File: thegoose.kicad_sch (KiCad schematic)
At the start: 31 parts, among them U1 DRV8848, U2 DRV8848, U3 DRV8848, U4 AP64500SP-13

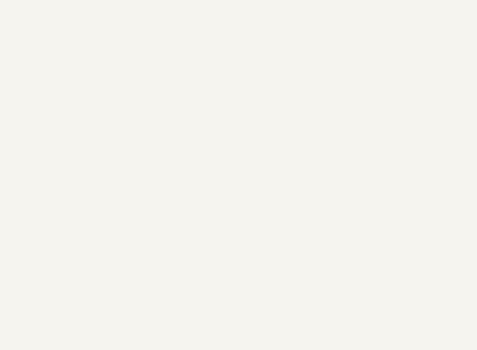
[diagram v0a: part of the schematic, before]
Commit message: Add LCSC part numbers
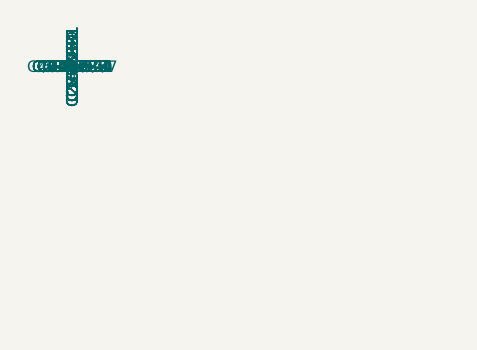
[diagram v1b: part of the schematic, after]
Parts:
- BT1: LCSC Part # (none) -> C98732
- C1: LCSC Part # (none) -> C106837
- C10, C15, C3, C6: LCSC Part # (none) -> C272880
- C11, C14, C4, C7: LCSC Part # (none) -> C344180
- C13, C2, C9: LCSC Part # (none) -> C76638
- C16: LCSC Part # (none) -> C1847101
- ESP32: LCSC Part # (none) -> C82899
- GPIO1: LCSC Part # (none) -> C42431837
- L1: LCSC Part # (none) -> C167779
- M1, M2, M3, M4, M5, M6: LCSC Part # (none) -> C157931
- R25: LCSC Part # (none) -> C844827
- R26: LCSC Part # (none) -> C5200544
- R27: LCSC Part # (none) -> C856785
- R28: LCSC Part # (none) -> C170028
- U1, U2, U3: LCSC Part # (none) -> C2863921
- U4: LCSC Part # (none) -> C2070920
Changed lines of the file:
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@@
 		(on_board yes)
 		(dnp no)
+		(property "LCSC Part #" "C344180")
 		(property "Reference" "C7"
 			(at 145.796 43.942 0)
@@
 		(dnp no)
 		(fields_autoplaced yes)
+		(property "LCSC Part #" "C272880")
 		(property "Reference" "C15"
 			(at 44.45 171.4499 0)
@@
 		(on_board yes)
 		(dnp no)
+		(property "LCSC Part #" "C157931")
 		(property "Reference" "M3"
 			(at 162.56 16.51 90)
@@
 		(on_board yes)
 		(dnp no)
+		(property "LCSC Part #" "C42431837")
 		(property "Reference" "GPIO1"
 			(at 102.362 95.758 0)
@@
 		(dnp no)
 		(fields_autoplaced yes)
+		(property "LCSC Part #" "C167779")
 		(property "Reference" "L1"
 			(at 82.55 158.75 90)
@@
 		(on_board yes)
 		(dnp no)
+		(property "LCSC Part #" "C82899")
 		(property "Reference" "ESP32"
 			(at 47.498 103.632 0)
@@
 		(on_board yes)
 		(dnp no)
+		(property "LCSC Part #" "C344180")
 		(property "Reference" "C11"
 			(at 74.676 43.942 0)
@@
 		(on_board yes)
 		(dnp no)
+		(property "LCSC Part #" "C844827")
 		(property "Reference" "R25"
 			(at 55.88 177.8 90)
@@
 		(on_board yes)
 		(dnp no)
+		(property "LCSC Part #" "C76638")
 		(property "Reference" "C2"
 			(at 225.552 21.844 0)
@@
 		(on_board yes)
 		(dnp no)
+		(property "LCSC Part #" "C2070920")
 		(property "Reference" "U4"
 			(at 64.77 164.592 0)
@@
 		(on_board yes)
 		(dnp no)
+		(property "LCSC Part #" "C5200544")
 		(property "Reference" "R26"
 			(at 101.6 167.64 90)
@@
 		(dnp no)
 		(fields_autoplaced yes)
+		(property "LCSC Part #" "C2863921")
 		(property "Reference" "U3"
 			(at 114.3 46.6246 90)
@@
 		(on_board yes)
 		(dnp no)
+		(property "LCSC Part #" "C98732")
 		(property "Reference" "BT1"
 			(at 39.37 158.75 0)
@@
 		(on_board yes)
 		(dnp no)
+		(property "LCSC Part #" "C157931")
 		(property "Reference" "M2"
 			(at 245.11 16.51 90)
@@
 		(on_board yes)
 		(dnp no)
+		(property "LCSC Part #" "C272880")
 		(property "Reference" "C6"
 			(at 129.794 34.798 0)
@@
 		(on_board yes)
 		(dnp no)
+		(property "LCSC Part #" "C106837")
 		(property "Reference" "C1"
 			(at 16.764 98.806 0)
@@
 		(on_board yes)
 		(dnp no)
+		(property "LCSC Part #" "C272880")
 		(property "Reference" "C10"
 			(at 58.674 34.798 0)
@@
 		(on_board yes)
 		(dnp no)
+		(property "LCSC Part #" "C344180")
 		(property "Reference" "C4"
 			(at 218.186 43.942 0)
@@
 		(on_board yes)
 		(dnp no)
+		(property "LCSC Part #" "C157931")
 		(property "Reference" "M4"
 			(at 172.72 16.51 90)
@@
 		(on_board yes)
 		(dnp no)
+		(property "LCSC Part #" "C157931")
 		(property "Reference" "M5"
 			(at 91.44 16.51 90)
@@
 		(on_board yes)
 		(dnp no)
+		(property "LCSC Part #" "C157931")
 		(property "Reference" "M1"
 			(at 234.95 16.51 90)
@@
 		(on_board yes)
 		(dnp no)
+		(property "LCSC Part #" "C157931")
 		(property "Reference" "M6"
 			(at 101.6 16.51 90)
@@
 		(on_board yes)
 		(dnp no)
+		(property "LCSC Part #" "C76638")
 		(property "Reference" "C9"
 			(at 153.162 21.844 0)
@@
 		(dnp no)
 		(fields_autoplaced yes)
+		(property "LCSC Part #" "C1847101")
 		(property "Reference" "C16"
 			(at 87.63 179.0699 0)
@@
 		(on_board yes)
 		(dnp no)
+		(property "LCSC Part #" "C76638")
 		(property "Reference" "C13"
 			(at 82.042 21.844 0)
@@
 		(on_board yes)
 		(dnp no)
+		(property "LCSC Part #" "C856785")
 		(property "Reference" "R27"
 			(at 101.6 175.26 90)
@@
 		(on_board yes)
 		(dnp no)
+		(property "LCSC Part #" "C272880")
 		(property "Reference" "C3"
 			(at 202.184 34.798 0)
@@
 		(on_board yes)
 		(dnp no)
+		(property "LCSC Part #" "C170028")
 		(property "Reference" "R28"
 			(at 87.63 172.72 90)
@@
 		(on_board yes)
 		(dnp no)
+		(property "LCSC Part #" "C344180")
 		(property "Reference" "C14"
 			(at 65.532 150.114 0)
@@
 		(dnp no)
 		(fields_autoplaced yes)
+		(property "LCSC Part #" "C2863921")
 		(property "Reference" "U2"
 			(at 185.42 46.6246 90)
@@
 		(dnp no)
 		(fields_autoplaced yes)
+		(property "LCSC Part #" "C2863921")
 		(property "Reference" "U1"
 			(at 257.81 46.6246 90)
